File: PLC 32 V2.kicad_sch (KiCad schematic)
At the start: 8 parts, among them J5 Screw_Terminal_01x10, J6 Screw_Terminal_01x02, J7 MODULO RTC, J8 Screw_Terminal_01x02, U18 ESP32-WROOM-32D

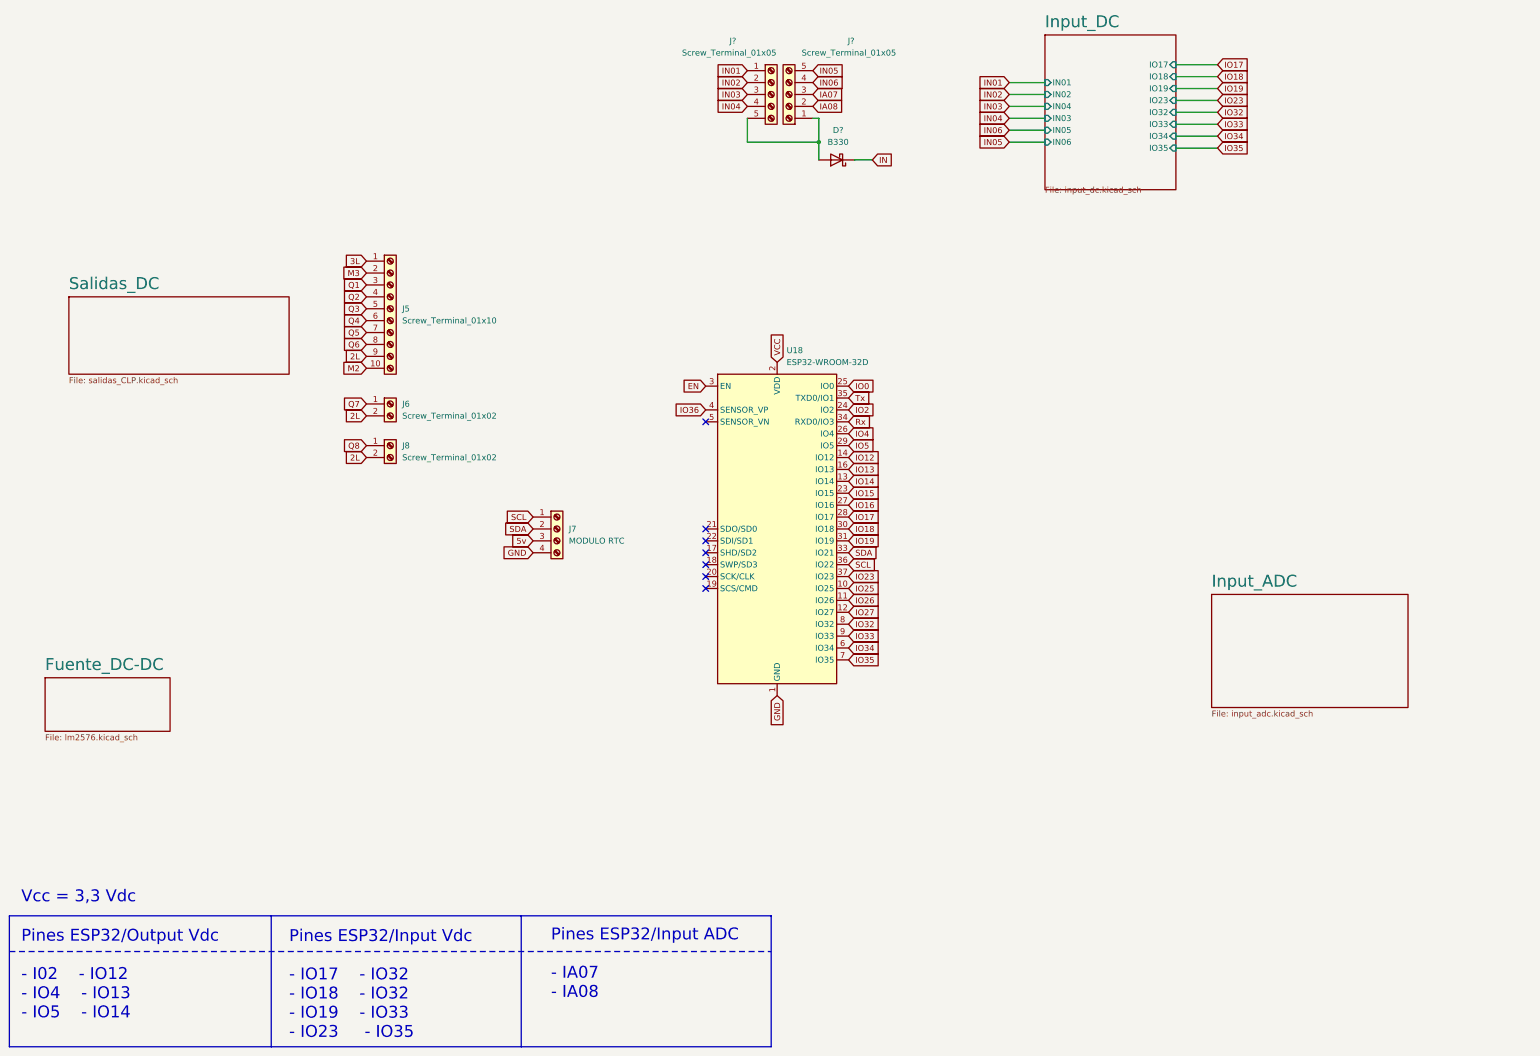
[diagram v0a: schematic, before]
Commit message: update esq raiz
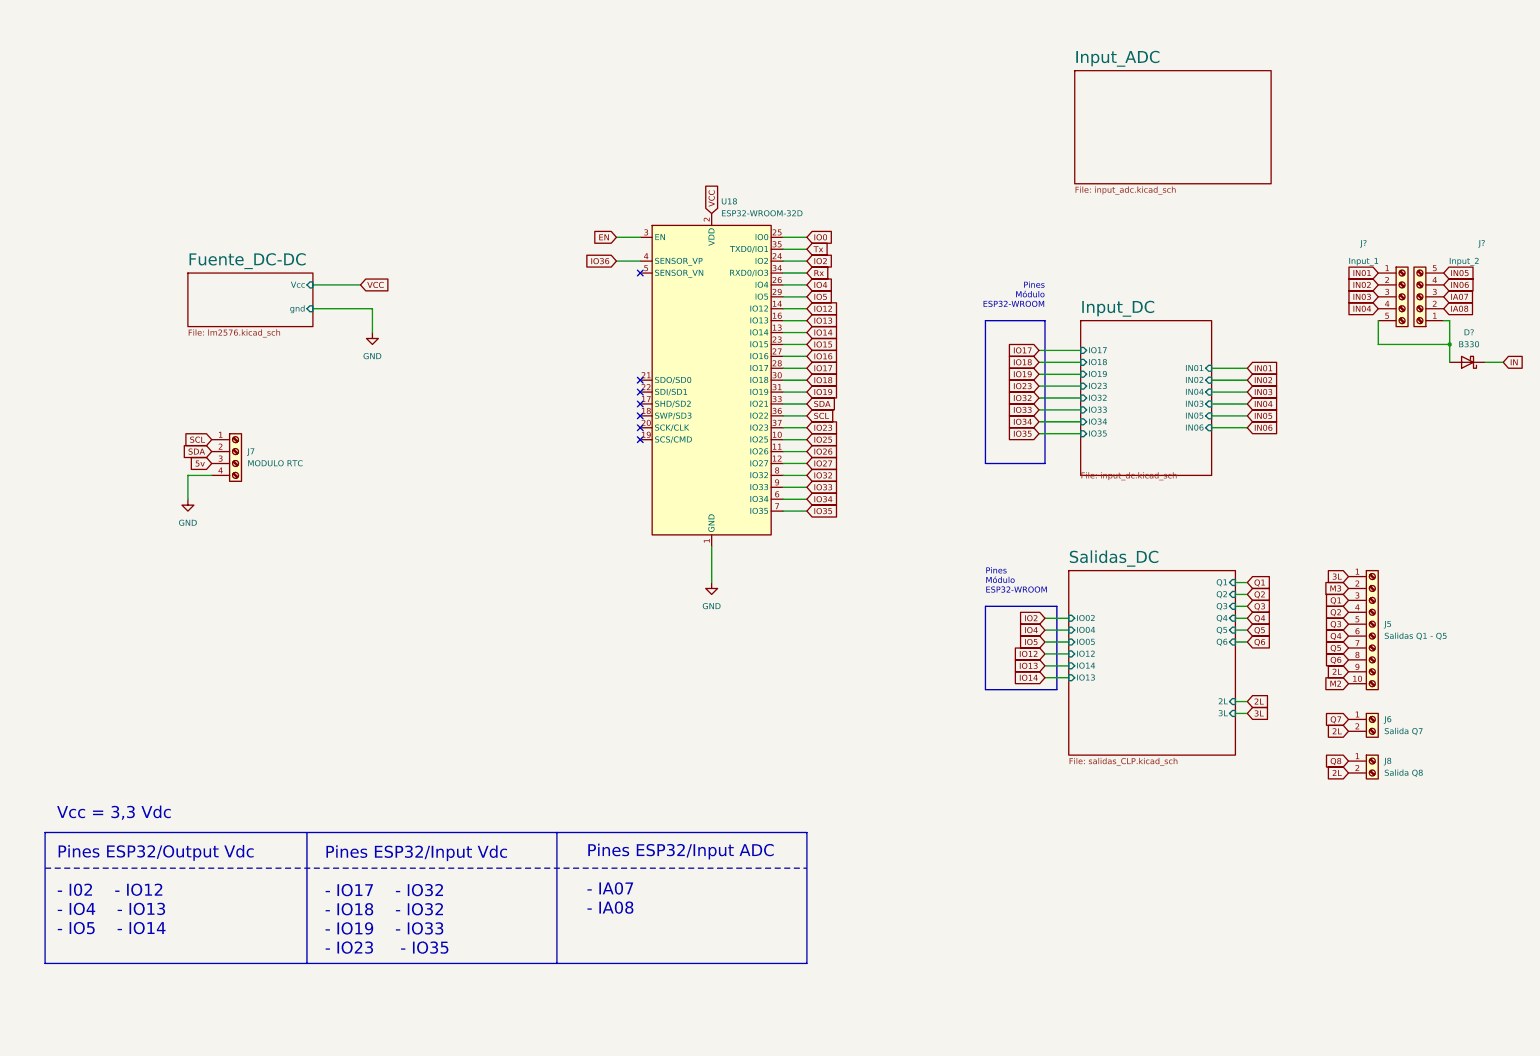
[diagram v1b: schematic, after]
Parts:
- J5: value Screw_Terminal_01x10 -> Salidas Q1 - Q5
- J6: value Screw_Terminal_01x02 -> Salida Q7
- J8: value Screw_Terminal_01x02 -> Salida Q8
- J?: value Screw_Terminal_01x05 -> Input_1
- J?: value Screw_Terminal_01x05 -> Input_2
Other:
- sheet Fuente_DC-DC ports: added Vcc, gnd; removed none
- sheet Salidas_DC ports: added 2L, 3L, IO02, IO04, IO05, IO12, IO13, IO14, Q1, Q2, Q3, Q4, Q5, Q6; removed none
- note added: "Pines Módulo ESP32-WROOM"
- moved on the sheet: D?, J5, J6, J7, J8, J?, U18

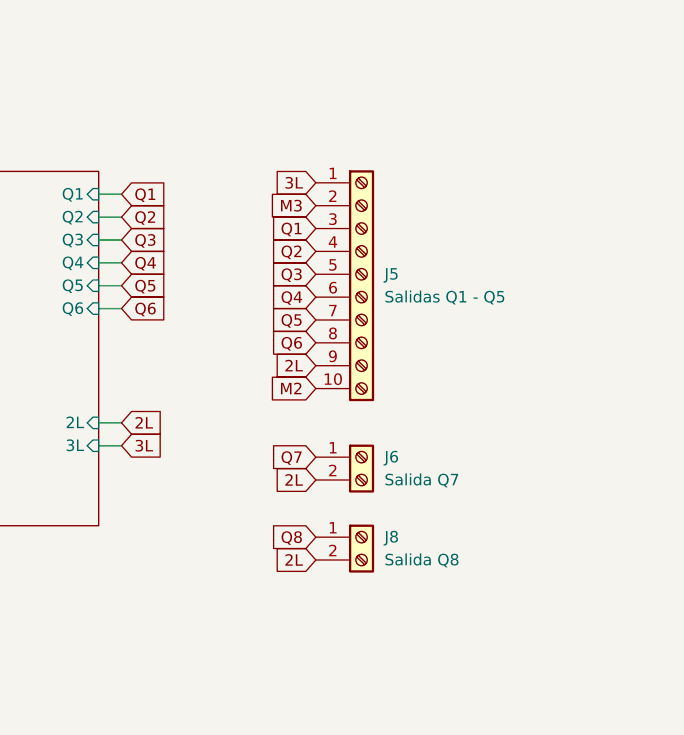
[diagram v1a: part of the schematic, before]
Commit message: update esq raiz salidas
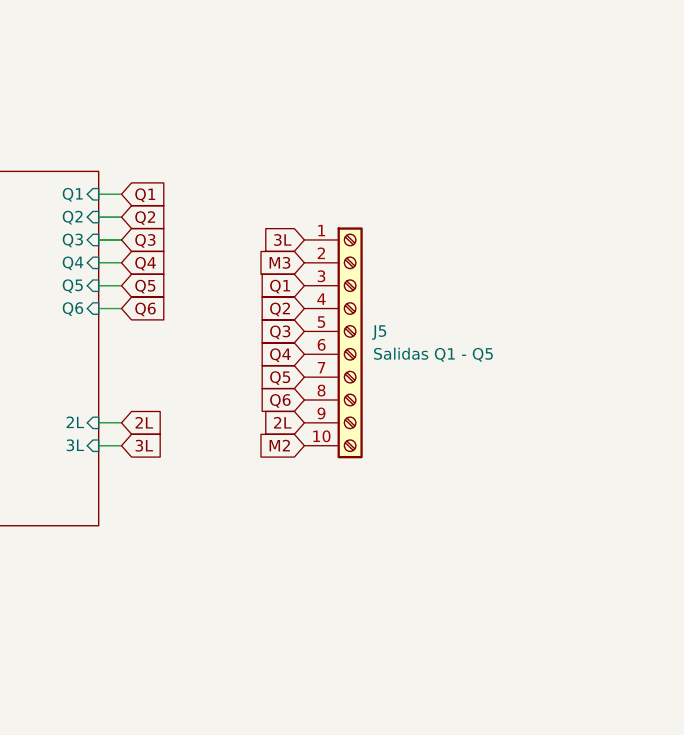
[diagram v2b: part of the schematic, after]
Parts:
- removed J6: Salida Q7, TerminalBlock:TerminalBlock_bornier-2_P5.08mm, symbol Connector:Screw_Terminal_01x02
- removed J8: Salida Q8, TerminalBlock:TerminalBlock_bornier-2_P5.08mm, symbol Connector:Screw_Terminal_01x02
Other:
- moved on the sheet: J5
